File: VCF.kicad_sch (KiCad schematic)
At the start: 57 parts, among them Q1 MMBF4393LT1G, Q2 MMBT3904-7-F, Q3 MMBT3906LT1G, Q4 MMBT3904-7-F, Q5 MMBT3906LT1G, Q6 MMBF4393LT1G, SW1 SW_SPST, SW2 SW_SPDT, U1 TL072, U2 LM13700

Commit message: more work...
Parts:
- C1, C2, C3, C4, C5: footprint Capacitor_SMD:C_0805_2012Metric_Pad1.18x1.45mm_HandSolder -> Capacitor_SMD:C_0805_2012Metric
- C10, C6, C7, C8, C9: footprint Capacitor_SMD:C_0805_2012Metric_Pad1.18x1.45mm_HandSolder -> Capacitor_SMD:C_0603_1608Metric
- R1, R10, R11, R12, R13, R14, R15, R16, R17, R18, R19, R2, R20, R21, R22, R23, R24, R25, R26, R27, R28, R29, R3, R4, R5, R6, R7, R8, R9: footprint Resistor_SMD:R_0805_2012Metric_Pad1.20x1.40mm_HandSolder -> Resistor_SMD:R_0603_1608Metric
- RV?: footprint Potentiometer_THT:Potentiometer_Alps_RK09K_Single_Vertical -> Potentiometer_SMD:Potentiometer_Bourns_TC33X_Vertical

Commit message: finishing schematic 1.0
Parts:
- SW1: footprint (none) -> SynthProjConnectors:MTS-103-A01-T0
- SW2: footprint SynthProjConnectors:ST-0-102-A01-T000-LF -> SynthProjConnectors:MTS-103-A01-T0

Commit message: Doing some layout
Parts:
- RV?: footprint Potentiometer_THT:Potentiometer_Alps_RK09K_Single_Vertical -> Potentiometer_SMD:Potentiometer_Bourns_TC33X_Vertical
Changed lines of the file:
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@@
       (effects (font (size 1.27 1.27)) (justify right))
     )
-    (property "Footprint" "Potentiometer_THT:Potentiometer_Alps_RK09K_Single_Vertical" (at 160.02 49.53 0)
+    (property "Footprint" "Potentiometer_SMD:Potentiometer_Bourns_TC33X_Vertical" (at 160.02 49.53 0)
       (effects (font (size 1.27 1.27)) hide)
     )

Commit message: lots of routes, added vco3, lfo2.
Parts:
- SW1, SW2: footprint SynthProjConnectors:MTS-103-A01-T0 -> SynthProjConnectors:SMTS-102
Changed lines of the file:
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@@
       (effects (font (size 1.27 1.27)))
     )
-    (property "Footprint" "SynthProjConnectors:MTS-103-A01-T0" (at 81.28 100.33 0)
+    (property "Footprint" "SynthProjConnectors:SMTS-102" (at 81.28 100.33 0)
       (effects (font (size 1.27 1.27)) hide)
     )
@@
       (effects (font (size 1.27 1.27)))
     )
-    (property "Footprint" "SynthProjConnectors:MTS-103-A01-T0" (at 254 127 0)
-      (effects (font (size 1.27 1.27)) hide)
-    )
+    (property "Footprint" "SynthProjConnectors:SMTS-102" (at 254 127 0)
+      (effects (font (size 1.27 1.27)) hide)
+    )

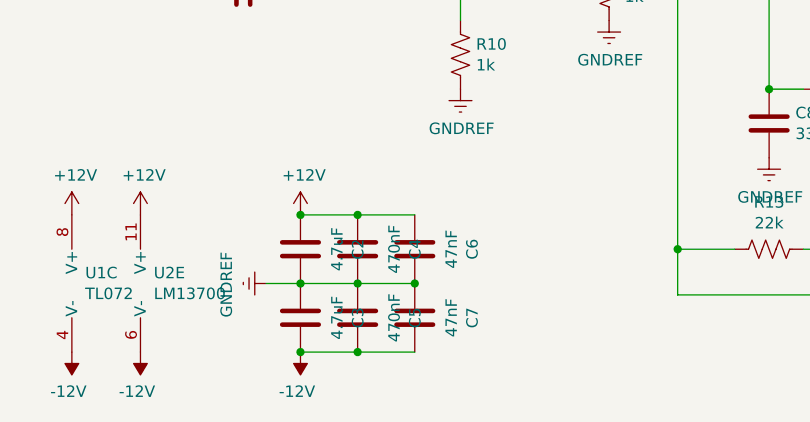
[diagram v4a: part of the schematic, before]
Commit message: more and more and more and more and more routing
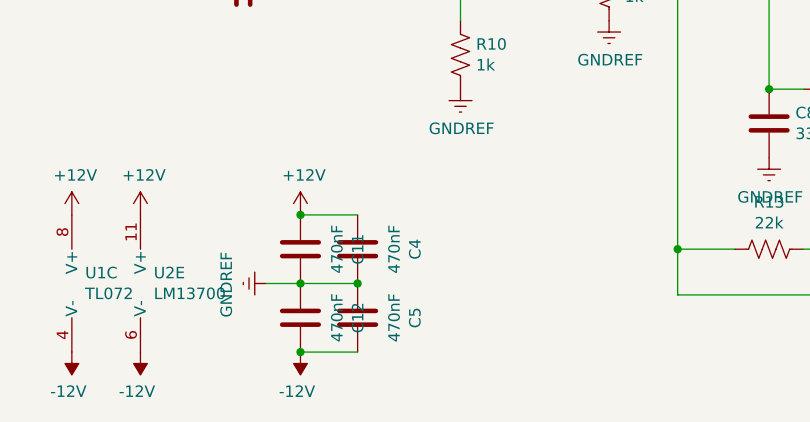
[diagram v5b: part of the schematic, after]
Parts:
- removed C2, C3: 4.7uF, Capacitor_SMD:C_0805_2012Metric, symbol Device:C
- removed C6, C7: 47nF, Capacitor_SMD:C_0603_1608Metric, symbol Device:C
- added C11, C12: 470nF, Capacitor_SMD:C_0805_2012Metric, symbol Device:C
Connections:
- net +12V: now also C11.2
- net -12V: now also C12.1
- net GNDREF: now also C11.1, C12.2
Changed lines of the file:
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@@
   (junction (at 241.3 116.84) (diameter 0) (color 0 0 0 0)
   )
+  (junction (at 85.09 160.02) (diameter 0) (color 0 0 0 0)
+  )
   (junction (at 173.99 138.43) (diameter 0) (color 0 0 0 0)
   )
+  (junction (at 165.1 138.43) (diameter 0) (color 0 0 0 0)
+  )
+  (junction (at 165.1 114.3) (diameter 0) (color 0 0 0 0)
+  )
+  (junction (at 106.68 88.9) (diameter 0) (color 0 0 0 0)
+  )
+  (junction (at 160.02 74.93) (diameter 0) (color 0 0 0 0)
+  )
+  (junction (at 71.12 35.56) (diameter 0) (color 0 0 0 0)
+  )
+  (junction (at 60.96 104.14) (diameter 0) (color 0 0 0 0)
+  )
+  (junction (at 241.3 138.43) (diameter 0) (color 0 0 0 0)
+  )
+  (junction (at 223.52 85.09) (diameter 0) (color 0 0 0 0)
+  )
+  (junction (at 102.87 127) (diameter 0) (color 0 0 0 0)
+  )
   (junction (at 85.09 152.4) (diameter 0) (color 0 0 0 0)
   )
-  (junction (at 165.1 138.43) (diameter 0) (color 0 0 0 0)
-  )
-  (junction (at 165.1 114.3) (diameter 0) (color 0 0 0 0)
-  )
-  (junction (at 106.68 88.9) (diameter 0) (color 0 0 0 0)
-  )
-  (junction (at 160.02 74.93) (diameter 0) (color 0 0 0 0)
-  )
-  (junction (at 85.09 160.02) (diameter 0) (color 0 0 0 0)
-  )
-  (junction (at 71.12 35.56) (diameter 0) (color 0 0 0 0)
-  )
-  (junction (at 60.96 104.14) (diameter 0) (color 0 0 0 0)
-  )
-  (junction (at 241.3 138.43) (diameter 0) (color 0 0 0 0)
-  )
-  (junction (at 223.52 85.09) (diameter 0) (color 0 0 0 0)
-  )
-  (junction (at 102.87 127) (diameter 0) (color 0 0 0 0)
-  )
   (junction (at 167.64 58.42) (diameter 0) (color 0 0 0 0)
   )
@@
   (junction (at 137.16 138.43) (diameter 0) (color 0 0 0 0)
   )
-  (junction (at 97.79 160.02) (diameter 0) (color 0 0 0 0)
-  )
   (junction (at 85.09 167.64) (diameter 0) (color 0 0 0 0)
   )
@@
   (junction (at 149.86 91.44) (diameter 0) (color 0 0 0 0)
   )
-  (junction (at 91.44 167.64) (diameter 0) (color 0 0 0 0)
-  )
   (junction (at 148.59 151.13) (diameter 0) (color 0 0 0 0)
   )
   (junction (at 167.64 66.04) (diameter 0) (color 0 0 0 0)
   )
-  (junction (at 91.44 152.4) (diameter 0) (color 0 0 0 0)
-  )
   (junction (at 106.68 66.04) (diameter 0) (color 0 0 0 0)
   )
@@
     (stroke (width 0) (type default))
   )
-  (wire (pts (xy 91.44 152.4) (xy 97.79 152.4))
-    (stroke (width 0) (type default))
-  )
   (wire (pts (xy 85.09 118.11) (xy 85.09 113.03))
     (stroke (width 0) (type default))
@@
     (stroke (width 0) (type default))
   )
+  (wire (pts (xy 85.09 160.02) (xy 91.44 160.02))
+    (stroke (width 0) (type default))
+  )
   (wire (pts (xy 190.5 116.84) (xy 190.5 114.3))
     (stroke (width 0) (type default))
@@
     (stroke (width 0) (type default))
   )
-  (wire (pts (xy 91.44 167.64) (xy 97.79 167.64))
-    (stroke (width 0) (type default))
-  )
   (wire (pts (xy 215.9 80.01) (xy 215.9 92.71))
     (stroke (width 0) (type default))
@@
     (stroke (width 0) (type default))
   )
-  (wire (pts (xy 85.09 160.02) (xy 91.44 160.02))
-    (stroke (width 0) (type default))
-  )
   (wire (pts (xy 133.35 100.33) (xy 133.35 93.98))
     (stroke (width 0) (type default))
@@
   )
   (wire (pts (xy 223.52 116.84) (xy 226.06 116.84))
-    (stroke (width 0) (type default))
-  )
-  (wire (pts (xy 91.44 160.02) (xy 97.79 160.02))
     (stroke (width 0) (type default))
   )
@@
     )
   )
+  (symbol (lib_id "Device:C") (at 91.44 156.21 180) (unit 1)
+    (in_bom yes) (on_board yes) (dnp no)
+    (property "Reference" "C4" (at 97.8408 156.21 90)
+      (effects (font (size 1.27 1.27)))
+    )
+    (property "Value" "470nF" (at 95.5294 156.21 90)
+      (effects (font (size 1.27 1.27)))
+    )
+    (property "Footprint" "Capacitor_SMD:C_0805_2012Metric" (at 90.4748 152.4 0)
+      (effects (font (size 1.27 1.27)) hide)
+    )
+    (property "Datasheet" "~" (at 91.44 156.21 0)
+      (effects (font (size 1.27 1.27)) hide)
+    )
+    (pin "2")
+    (pin "1")
+    (instances
+      (project "SynthProj"
+        (path "/9021c97e-351f-4ed9-b393-50257df6a463/00000000-0000-0000-0000-0000659a4e2e"
+          (reference "C4") (unit 1)
+        )
+      )
+    )
+  )
+  (symbol (lib_id "Device:C") (at 91.44 163.83 180) (unit 1)
+    (in_bom yes) (on_board yes) (dnp no)
+    (property "Reference" "C5" (at 97.8408 163.83 90)
+      (effects (font (size 1.27 1.27)))
+    )
+    (property "Value" "470nF" (at 95.5294 163.83 90)
+      (effects (font (size 1.27 1.27)))
+    )
+    (property "Footprint" "Capacitor_SMD:C_0805_2012Metric" (at 90.4748 160.02 0)
+      (effects (font (size 1.27 1.27)) hide)
+    )
+    (property "Datasheet" "~" (at 91.44 163.83 0)
+      (effects (font (size 1.27 1.27)) hide)
+    )
+    (pin "1")
+    (pin "2")
+    (instances
+      (project "SynthProj"
+        (path "/9021c97e-351f-4ed9-b393-50257df6a463/00000000-0000-0000-0000-0000659a4e2e"
+          (reference "C5") (unit 1)
+        )
+      )
+    )
+  )
   (symbol (lib_id "Device:C") (at 85.09 156.21 180) (unit 1)
     (in_bom yes) (on_board yes) (dnp no)
-    (property "Reference" "C2" (at 91.4908 156.21 90)
-      (effects (font (size 1.27 1.27)))
-    )
-    (property "Value" "4.7uF" (at 89.1794 156.21 90)
+    (property "Reference" "C11" (at 91.4908 156.21 90)
+      (effects (font (size 1.27 1.27)))
+    )
+    (property "Value" "470nF" (at 89.1794 156.21 90)
       (effects (font (size 1.27 1.27)))
     )
@@
       (project "SynthProj"
         (path "/9021c97e-351f-4ed9-b393-50257df6a463/00000000-0000-0000-0000-0000659a4e2e"
-          (reference "C2") (unit 1)
-        )
-      )
-    )
-  )
-  (symbol (lib_id "Device:C") (at 91.44 156.21 180) (unit 1)
-    (in_bom yes) (on_board yes) (dnp no)
-    (property "Reference" "C4" (at 97.8408 156.21 90)
-      (effects (font (size 1.27 1.27)))
-    )
-    (property "Value" "470nF" (at 95.5294 156.21 90)
-      (effects (font (size 1.27 1.27)))
-    )
-    (property "Footprint" "Capacitor_SMD:C_0805_2012Metric" (at 90.4748 152.4 0)
-      (effects (font (size 1.27 1.27)) hide)
-    )
-    (property "Datasheet" "~" (at 91.44 156.21 0)
-      (effects (font (size 1.27 1.27)) hide)
-    )
-    (pin "2")
-    (pin "1")
-    (instances
-      (project "SynthProj"
-        (path "/9021c97e-351f-4ed9-b393-50257df6a463/00000000-0000-0000-0000-0000659a4e2e"
-          (reference "C4") (unit 1)
-        )
-      )
-    )
-  )
-  (symbol (lib_id "Device:C") (at 97.79 156.21 180) (unit 1)
-    (in_bom yes) (on_board yes) (dnp no)
-    (property "Reference" "C6" (at 104.1908 156.21 90)
-      (effects (font (size 1.27 1.27)))
-    )
-    (property "Value" "47nF" (at 101.8794 156.21 90)
-      (effects (font (size 1.27 1.27)))
-    )
-    (property "Footprint" "Capacitor_SMD:C_0603_1608Metric" (at 96.8248 152.4 0)
-      (effects (font (size 1.27 1.27)) hide)
-    )
-    (property "Datasheet" "~" (at 97.79 156.21 0)
-      (effects (font (size 1.27 1.27)) hide)
-    )
-    (pin "1")
-    (pin "2")
-    (instances
-      (project "SynthProj"
-        (path "/9021c97e-351f-4ed9-b393-50257df6a463/00000000-0000-0000-0000-0000659a4e2e"
-          (reference "C6") (unit 1)
+          (reference "C11") (unit 1)
         )
       )
@@
   (symbol (lib_id "Device:C") (at 85.09 163.83 180) (unit 1)
     (in_bom yes) (on_board yes) (dnp no)
-    (property "Reference" "C3" (at 91.4908 163.83 90)
-      (effects (font (size 1.27 1.27)))
-    )
-    (property "Value" "4.7uF" (at 89.1794 163.83 90)
+    (property "Reference" "C12" (at 91.4908 163.83 90)
+      (effects (font (size 1.27 1.27)))
+    )
+    (property "Value" "470nF" (at 89.1794 163.83 90)
       (effects (font (size 1.27 1.27)))
     )
@@
       (project "SynthProj"
         (path "/9021c97e-351f-4ed9-b393-50257df6a463/00000000-0000-0000-0000-0000659a4e2e"
-          (reference "C3") (unit 1)
-        )
-      )
-    )
-  )
-  (symbol (lib_id "Device:C") (at 91.44 163.83 180) (unit 1)
-    (in_bom yes) (on_board yes) (dnp no)
-    (property "Reference" "C5" (at 97.8408 163.83 90)
-      (effects (font (size 1.27 1.27)))
-    )
-    (property "Value" "470nF" (at 95.5294 163.83 90)
-      (effects (font (size 1.27 1.27)))
-    )
-    (property "Footprint" "Capacitor_SMD:C_0805_2012Metric" (at 90.4748 160.02 0)
-      (effects (font (size 1.27 1.27)) hide)
-    )
-    (property "Datasheet" "~" (at 91.44 163.83 0)
-      (effects (font (size 1.27 1.27)) hide)
-    )
-    (pin "1")
-    (pin "2")
-    (instances
-      (project "SynthProj"
-        (path "/9021c97e-351f-4ed9-b393-50257df6a463/00000000-0000-0000-0000-0000659a4e2e"
-          (reference "C5") (unit 1)
-        )
-      )
-    )
-  )
-  (symbol (lib_id "Device:C") (at 97.79 163.83 180) (unit 1)
-    (in_bom yes) (on_board yes) (dnp no)
-    (property "Reference" "C7" (at 104.1908 163.83 90)
-      (effects (font (size 1.27 1.27)))
-    )
-    (property "Value" "47nF" (at 101.8794 163.83 90)
-      (effects (font (size 1.27 1.27)))
-    )
-    (property "Footprint" "Capacitor_SMD:C_0603_1608Metric" (at 96.8248 160.02 0)
-      (effects (font (size 1.27 1.27)) hide)
-    )
-    (property "Datasheet" "~" (at 97.79 163.83 0)
-      (effects (font (size 1.27 1.27)) hide)
-    )
-    (pin "2")
-    (pin "1")
-    (instances
-      (project "SynthProj"
-        (path "/9021c97e-351f-4ed9-b393-50257df6a463/00000000-0000-0000-0000-0000659a4e2e"
-          (reference "C7") (unit 1)
-        )
-      )
+          (reference "C12") (unit 1)
+        )
+      )
